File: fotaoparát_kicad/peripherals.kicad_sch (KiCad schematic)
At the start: 7 parts, among them J13 Micro_SD_Card_Det2

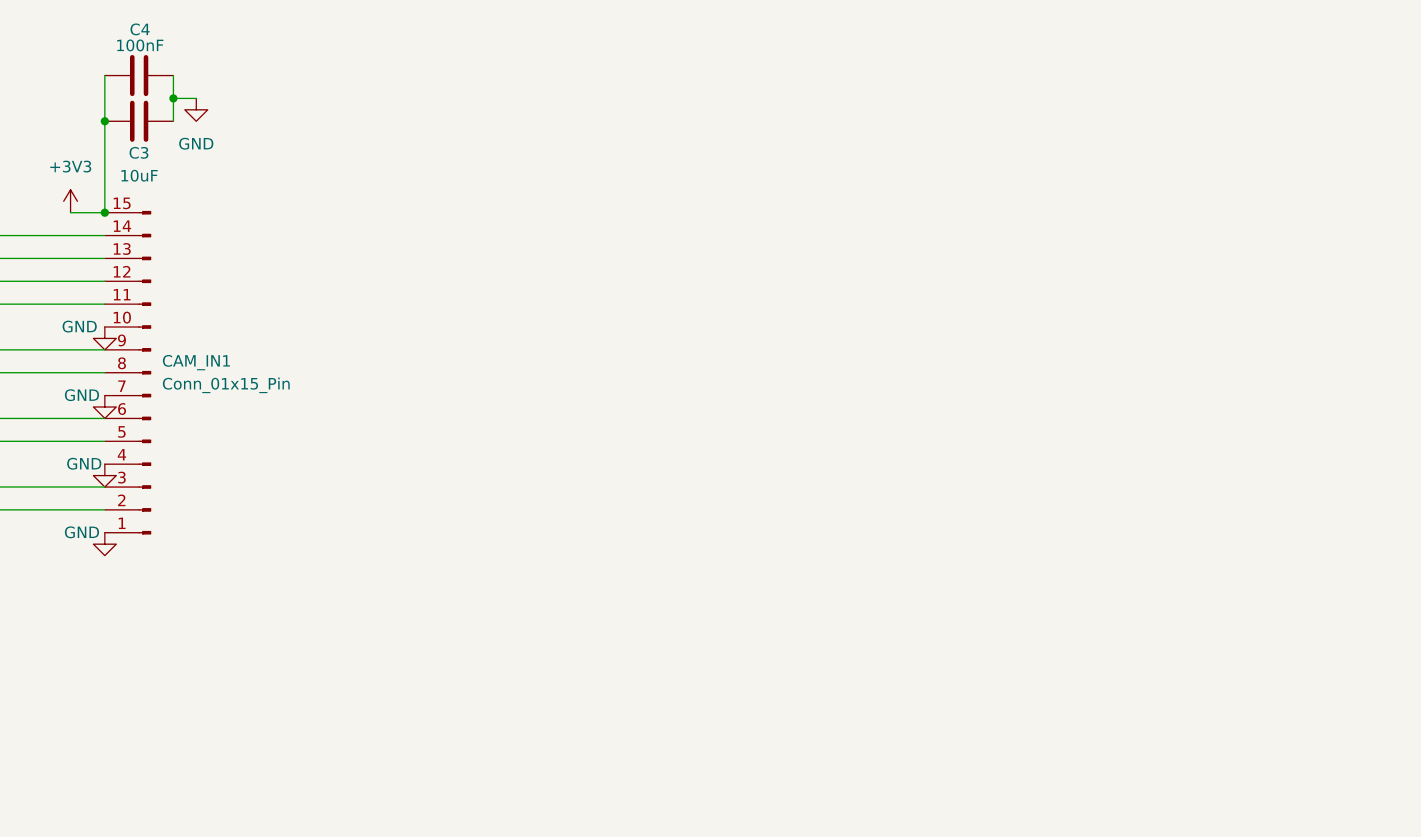
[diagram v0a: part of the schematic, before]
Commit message: Pridani konektoru pro tlacitka na schema
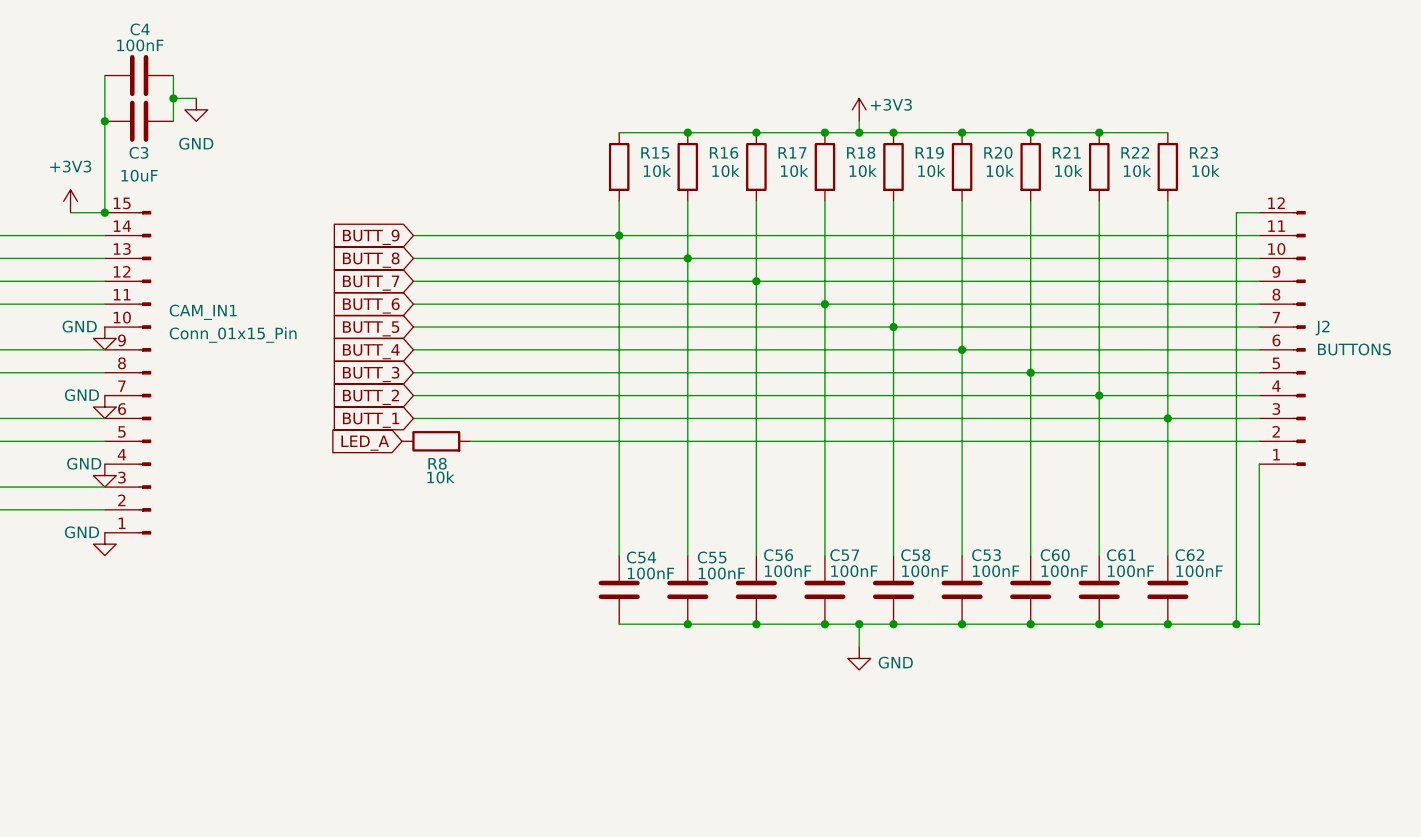
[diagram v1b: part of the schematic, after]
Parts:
- added C53, C54, C55, C56, C57, C58, C60, C61, C62: 100nF, Capacitor_SMD:C_0201_0603Metric, symbol Device:C
- added J2: BUTTONS, Connector_FFC-FPC:Hirose_FH12-12S-0.5SH_1x12-1MP_P0.50mm_Horizontal, symbol Connector:Conn_01x12_Pin
- added R15, R16, R17, R18, R19, R20, R21, R22, R23, R8: 10k, Resistor_SMD:R_0603_1608Metric, symbol Device:R
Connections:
- net +3V3: now also R15.1, R16.1, R17.1, R18.1, R19.1, R20.1, R21.1, R22.1, R23.1
- net GND: now also C53.2, C54.2, C55.2, C56.2, C57.2, C58.2, C60.2, C61.2, C62.2, J2.1 (Pin_1), J2.12 (Pin_12)
- new net: J2.2 (Pin_2), R8.2
- new net BUTT_1: C62.1, J2.3 (Pin_3), R23.2
- new net BUTT_2: C61.1, J2.4 (Pin_4), R22.2
- new net BUTT_3: C60.1, J2.5 (Pin_5), R21.2
- new net BUTT_4: C53.1, J2.6 (Pin_6), R20.2
- new net BUTT_5: C58.1, J2.7 (Pin_7), R19.2
- new net BUTT_6: C57.1, J2.8 (Pin_8), R18.2
- new net BUTT_7: C56.1, J2.9 (Pin_9), R17.2
- new net BUTT_8: C55.1, J2.10 (Pin_10), R16.2
- new net BUTT_9: C54.1, J2.11 (Pin_11), R15.2
- new net LED_A: R8.1
